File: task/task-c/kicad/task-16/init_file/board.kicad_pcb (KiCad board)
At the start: 2 copper layers, 100 x 72 mm, 3 parts, among them U1 OPAMP, U2 MCU

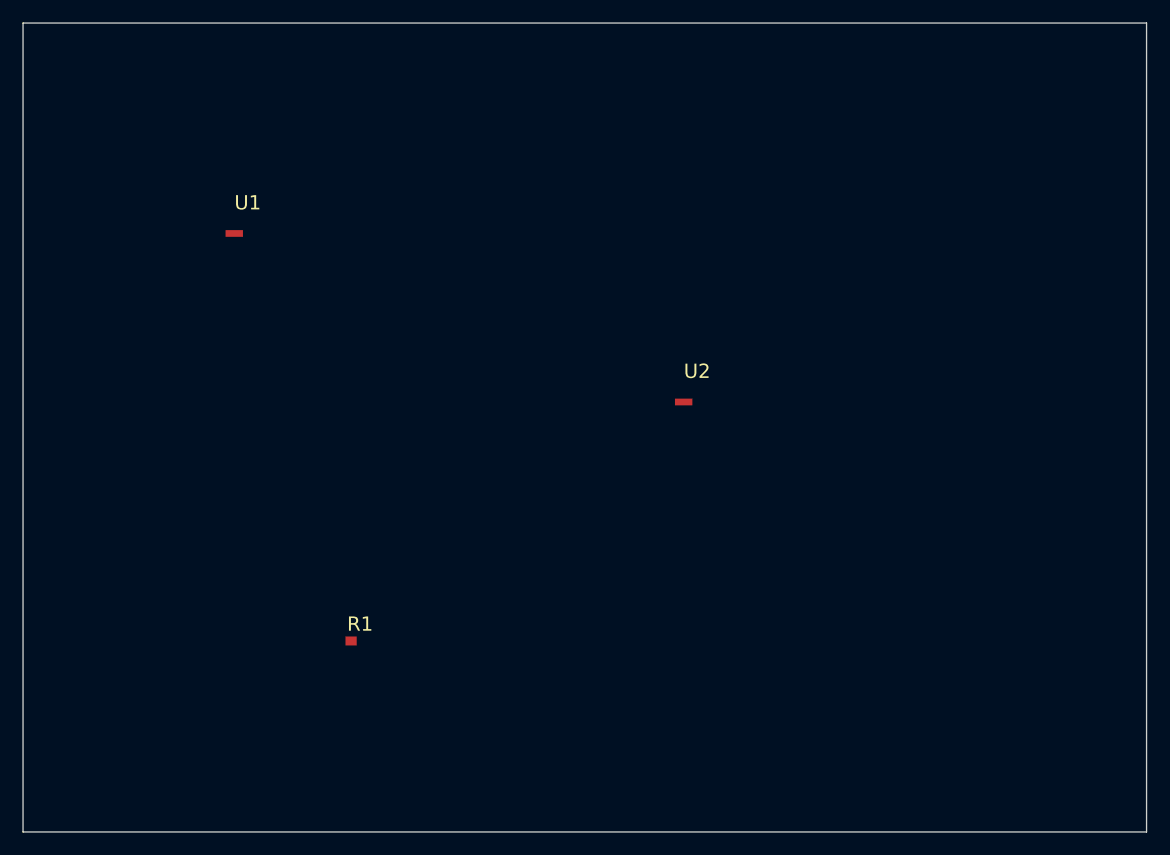
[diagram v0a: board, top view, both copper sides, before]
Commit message: Refine engineering task metadata and instructions
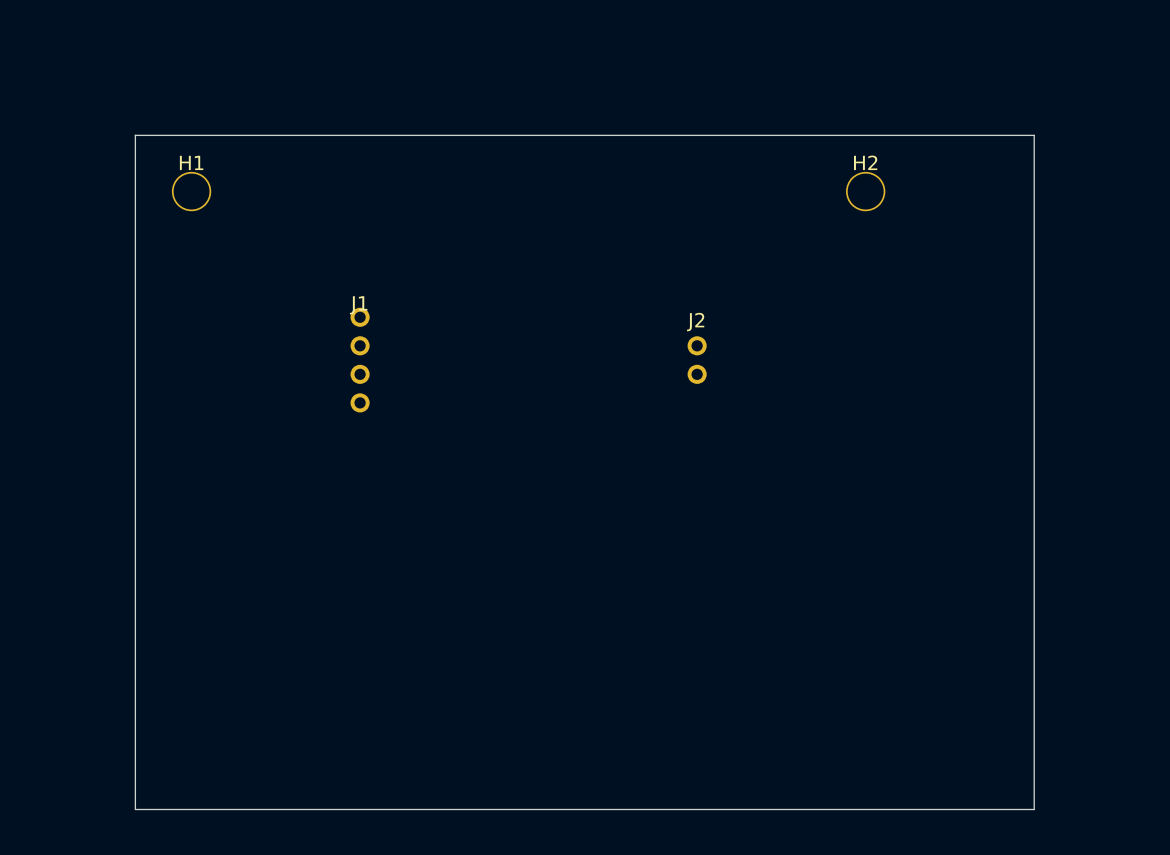
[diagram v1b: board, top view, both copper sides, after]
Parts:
- removed R1: 10k, Resistor_SMD:R_0603_1608Metric
- removed U1: OPAMP, Package_SO:SOIC-8_3.9x4.9mm_P1.27mm
- removed U2: MCU, Package_SO:SOIC-8_3.9x4.9mm_P1.27mm
- added H1: MH, MountingHole:MountingHole_3.2mm_M3, F.Cu at (15.0, 15.0)
- added H2: MH, MountingHole:MountingHole_3.2mm_M3, F.Cu at (75.0, 15.0)
- added J1: HDR_4, Connector_PinHeader_2.54mm:PinHeader_1x04_P2.54mm_Vertical, F.Cu at (30.0, 30.0)
- added J2: HDR_2, Connector_PinHeader_2.54mm:PinHeader_1x02_P2.54mm_Vertical, F.Cu at (60.0, 30.0)
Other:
- board size 100 x 72 mm -> 80 x 60 mm
- rule pad_to_mask_clearance: 0.1 -> 0.051
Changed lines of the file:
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@@
-(kicad_pcb
-  (version 20240108)
-  (generator "pcbnew")
-  (generator_version "9.0")
-  (general
-    (thickness 1.6)
-    (legacy_teardrops no)
-  )
+(kicad_pcb (version 20240108) (generator "pcbnew") (generator_version "9.0")
+  (general (thickness 1.6) (legacy_teardrops no))
   (paper "A4")
   (layers
@@
   )
   (setup
-    (pad_to_mask_clearance 0.1)
-    (allow_soldermask_bridges_in_footprints no)
+    (pad_to_mask_clearance 0.051)
   )
   (net 0 "")
-  (net 1 "VCC")
-  (net 2 "GND")
-  (gr_line (start 0 0) (end 100 0) (layer "Edge.Cuts") (stroke (width 0.1) (type solid)))
-  (gr_line (start 100 0) (end 100 72) (layer "Edge.Cuts") (stroke (width 0.1) (type solid)))
-  (gr_line (start 100 72) (end 0 72) (layer "Edge.Cuts") (stroke (width 0.1) (type solid)))
-  (gr_line (start 0 72) (end 0 0) (layer "Edge.Cuts") (stroke (width 0.1) (type solid)))
-  (footprint "Package_SO:SOIC-8_3.9x4.9mm_P1.27mm"
-    (layer "F.Cu")
-    (at 20 20)
-    (fp_text reference "U1" (at 0 -4) (layer "F.SilkS"))
-    (fp_text value "OPAMP" (at 0 4) (layer "F.Fab"))
-    (pad "1" smd rect (at -1.2 -1.27) (size 1.55 0.6) (layers "F.Cu" "F.Paste" "F.Mask") (net 1 "VCC"))
+  (net 1 "GND")
+  (net 2 "VCC")
+  (footprint "Connector_PinHeader_2.54mm:PinHeader_1x04_P2.54mm_Vertical" (layer "F.Cu") (at 30 30)
+    (property "Reference" "J1" (at 0 -5) (layer "F.SilkS"))
+    (property "Value" "HDR_4" (at 0 5) (layer "F.Fab"))
+    (pad "1" thru_hole circle (at 0 -3.81) (size 1.7 1.7) (drill 1.0) (layers "*.Cu" "*.Mask") (net 1 "GND"))
+    (pad "2" thru_hole circle (at 0 -1.27) (size 1.7 1.7) (drill 1.0) (layers "*.Cu" "*.Mask") (net 2 "VCC"))
+    (pad "3" thru_hole circle (at 0  1.27) (size 1.7 1.7) (drill 1.0) (layers "*.Cu" "*.Mask") (net 1 "GND"))
+    (pad "4" thru_hole circle (at 0  3.81) (size 1.7 1.7) (drill 1.0) (layers "*.Cu" "*.Mask") (net 2 "VCC"))
   )
-  (footprint "Package_SO:SOIC-8_3.9x4.9mm_P1.27mm"
-    (layer "F.Cu")
-    (at 60 35)
-    (fp_text reference "U2" (at 0 -4) (layer "F.SilkS"))
-    (fp_text value "MCU" (at 0 4) (layer "F.Fab"))
-    (pad "1" smd rect (at -1.2 -1.27) (size 1.55 0.6) (layers "F.Cu" "F.Paste" "F.Mask") (net 2 "GND"))
+  (footprint "Connector_PinHeader_2.54mm:PinHeader_1x02_P2.54mm_Vertical" (layer "F.Cu") (at 60 30)
+    (property "Reference" "J2" (at 0 -3.5) (layer "F.SilkS"))
+    (property "Value" "HDR_2" (at 0 3.5) (layer "F.Fab"))
+    (pad "1" thru_hole circle (at 0 -1.27) (size 1.7 1.7) (drill 1.0) (layers "*.Cu" "*.Mask") (net 1 "GND"))
+    (pad "2" thru_hole circle (at 0  1.27) (size 1.7 1.7) (drill 1.0) (layers "*.Cu" "*.Mask") (net 2 "VCC"))
   )
-  (footprint "Resistor_SMD:R_0603_1608Metric"
-    (layer "F.Cu")
-    (at 30 55)
-    (fp_text reference "R1" (at 0 -1.5) (layer "F.SilkS"))
-    (fp_text value "10k" (at 0 1.5) (layer "F.Fab"))
-    (pad "1" smd rect (at -0.8 0) (size 1.0 0.8) (layers "F.Cu" "F.Paste" "F.Mask") (net 1 "VCC"))
+  (footprint "MountingHole:MountingHole_3.2mm_M3" (layer "F.Cu") (at 15 15)
+    (property "Reference" "H1" (at 0 -2.5) (layer "F.SilkS"))
+    (property "Value" "MH" (at 0 2.5) (layer "F.Fab"))
+    (pad "" thru_hole circle (at 0 0) (size 3.5 3.5) (drill 3.2) (layers "*.Cu" "*.Mask"))
   )
+  (footprint "MountingHole:MountingHole_3.2mm_M3" (layer "F.Cu") (at 75 15)
+    (property "Reference" "H2" (at 0 -2.5) (layer "F.SilkS"))
+    (property "Value" "MH" (at 0 2.5) (layer "F.Fab"))
+    (pad "" thru_hole circle (at 0 0) (size 3.5 3.5) (drill 3.2) (layers "*.Cu" "*.Mask"))
+  )
+  (gr_line (start 10 10) (end 90 10) (layer "Edge.Cuts") (stroke (width 0.05) (type solid)))
+  (gr_line (start 90 10) (end 90 70) (layer "Edge.Cuts") (stroke (width 0.05) (type solid)))
+  (gr_line (start 90 70) (end 10 70) (layer "Edge.Cuts") (stroke (width 0.05) (type solid)))
+  (gr_line (start 10 70) (end 10 10) (layer "Edge.Cuts") (stroke (width 0.05) (type solid)))
 )
